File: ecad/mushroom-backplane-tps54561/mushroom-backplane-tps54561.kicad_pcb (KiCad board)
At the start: 2 copper layers, 24 x 63 mm, 43 parts, among them J1 BUSOUT, J2 BUSIN, J3 BACKPLANE, M1 KK 254, Q1 AO3400A, Q2 SI2301CDS-T1-GE3, U1 TPS54561

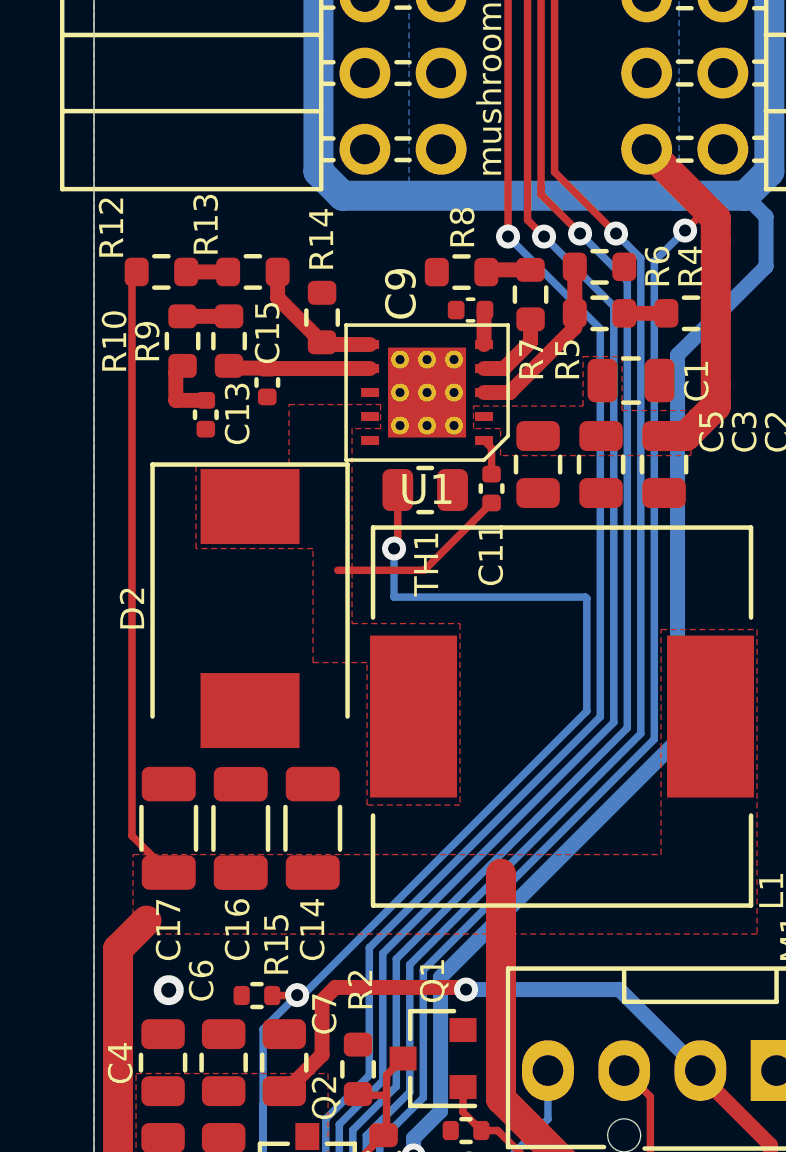
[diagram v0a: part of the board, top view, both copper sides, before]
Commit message: Organize ECAD files
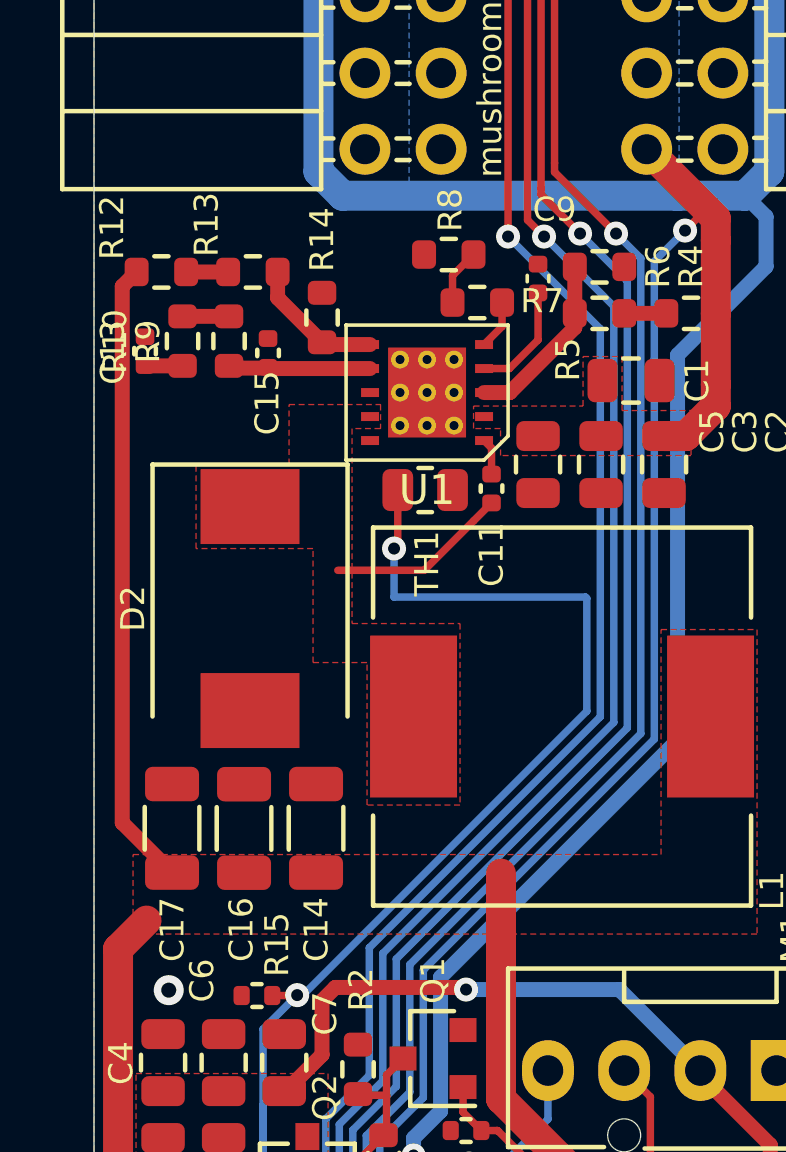
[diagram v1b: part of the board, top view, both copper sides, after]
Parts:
- U1: footprint Mycelium:WSON-10-1EP_4x4mm_P0.8_EP2.6x3.0mm -> mykilio:WSON-10-1EP_4x4mm_P0.8_EP2.6x3.0mm
- moved C13 2.93 mm to (89.7, 96.8), turned to 90 degrees
- moved C9 2.48 mm to (102.8, 94.4), turned to 90 degrees
- moved R7 1.79 mm to (100.8, 95.2), turned to 180 degrees
- moved C15 0.99 mm to (93.8, 96.9), turned to 90 degrees
- moved R8 0.72 mm to (99.8, 93.6)
- moved C14 0.11 mm to (95.4, 112.7)
- moved C16 0.11 mm to (93.0, 112.7)
- moved C17 0.11 mm to (90.6, 112.7)
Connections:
- U1 pad 4: Net-(R7-Pad1) -> Net-(C9-Pad1)
- U1 pad 5: Net-(C9-Pad1) -> Net-(R7-Pad1)
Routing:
- net Net-(C9-Pad1): track 1.28 -> 3.76 mm
- net Net-(R7-Pad1): track 2.67 -> 1.65 mm
- net Net-(C13-Pad1): track 2.31 -> 1.32 mm
- net 5VSMPS: track 53.5 -> 54.0 mm
